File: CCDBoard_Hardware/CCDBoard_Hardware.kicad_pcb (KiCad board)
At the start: 2 copper layers, 63.5 x 38.1 mm, 30 parts, among them U1 S11639-01, U2 LT1818, U3 74HC541

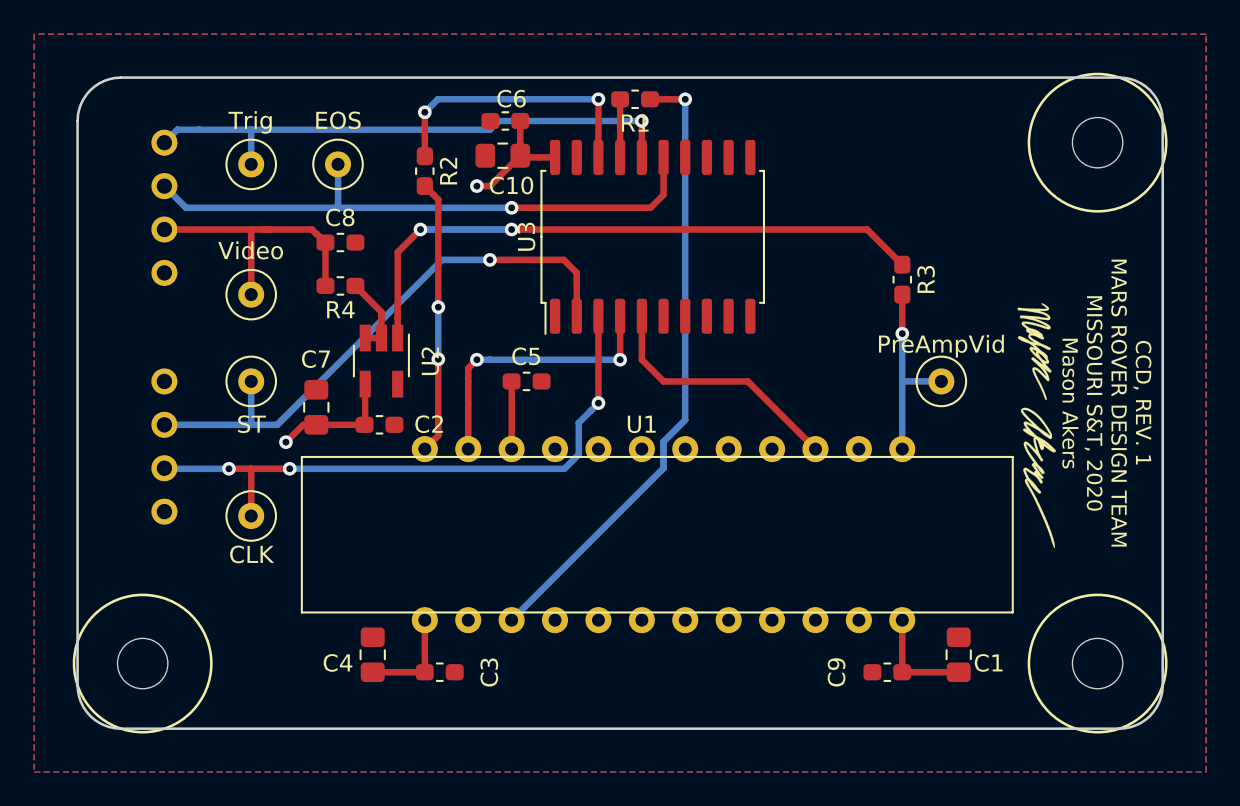
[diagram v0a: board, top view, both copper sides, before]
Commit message: improvements that might break things
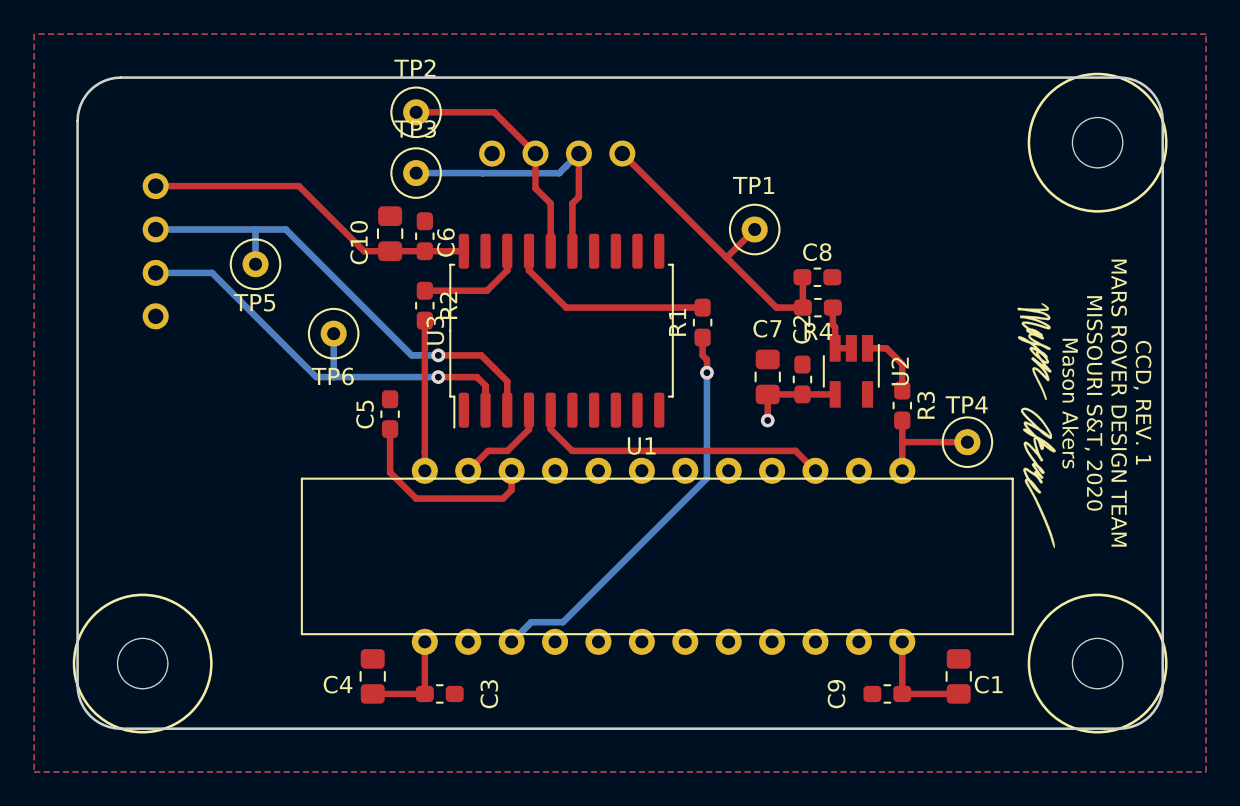
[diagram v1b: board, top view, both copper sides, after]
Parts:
- moved TP1 29.7 mm to (141.2, 85.1)
- moved C8 28.0 mm to (144.9, 87.9)
- moved R4 28.0 mm to (144.9, 89.7)
- moved U2 27.5 mm to (146.9, 93.4)
- moved C7 26.5 mm to (142.0, 93.7)
- moved C2 24.9 mm to (144.0, 93.9), turned to 90 degrees
- moved Conn2 23.2 mm to (129.7, 80.6), turned to 180 degrees
- moved TP5 14.7 mm to (112.0, 87.1)
- moved R1 13.7 mm to (138.2, 90.5), turned to 90 degrees
- moved Conn1 11.4 mm to (106.2, 86.4)
- moved TP2 10.1 mm to (121.4, 78.2)
- moved C6 8.23 mm to (121.9, 85.5), turned to 90 degrees
- moved C5 8.21 mm to (119.9, 95.9), turned to 90 degrees
- moved C10 8.02 mm to (119.9, 85.3), turned to 90 degrees
- moved R2 7.87 mm to (121.9, 89.5)
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- renumbered Video to TP1, Trig to TP2, EOS to TP3, PreAmpVid to TP4, CLK to TP5, ST to TP6
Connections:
- Conn1 pad 2: ST -> CLK
- Conn1 pad 3: CLK -> ST
- Conn2 pad 1: Trig -> Video
- Conn2 pad 3: Video -> Trig
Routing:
- net Net-(R3-Pad1): track 36.0 -> 3.97 mm, vias 2 -> 0
- net EOS: track 34.8 -> 15.9 mm, vias 1 -> 0
- net Trig: track 32.6 -> 14.1 mm, vias 1 -> 0
- net Net-(R1-Pad1): track 36.7 -> 23.7 mm
- net Trig_OUT: track 16.4 -> 5.69 mm, vias 2 -> 0
- net +5V: track 27.2 -> 37.5 mm, vias 2 -> 1
- net ST_IN: track 16.4 -> 6.44 mm, vias 2 -> 0
- net ST: track 35.7 -> 26.0 mm
- net CLK_IN: track 3.40 -> 12.2 mm
- net CLK: track 35.9 -> 28.0 mm, vias 3 -> 1
- net Net-(C5-Pad1): track 3.96 -> 11.6 mm
- net Net-(R2-Pad2): track 16.0 -> 8.79 mm, vias 2 -> 0
- net Net-(R3-Pad2): track 11.3 -> 6.75 mm, vias 1 -> 0
- net EOS_OUT: track 14.9 -> 17.6 mm
- net Video: track 16.3 -> 18.4 mm
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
